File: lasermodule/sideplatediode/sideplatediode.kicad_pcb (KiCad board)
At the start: 2 copper layers, 117 x 33.2 mm, 8 parts, among them J1 Conn_01x02, J2 Conn_01x01, J3 Conn_01x01, J4 Conn_01x01, J5 Conn_01x01

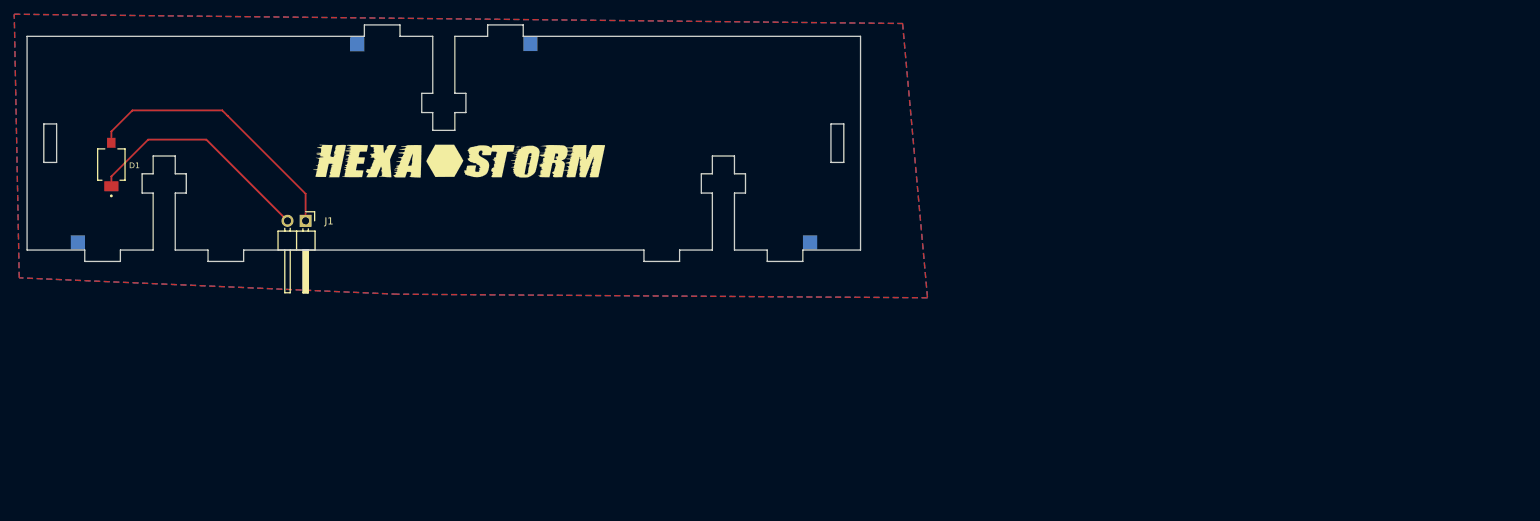
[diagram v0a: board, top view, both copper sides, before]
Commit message: board almost fully synced close for release
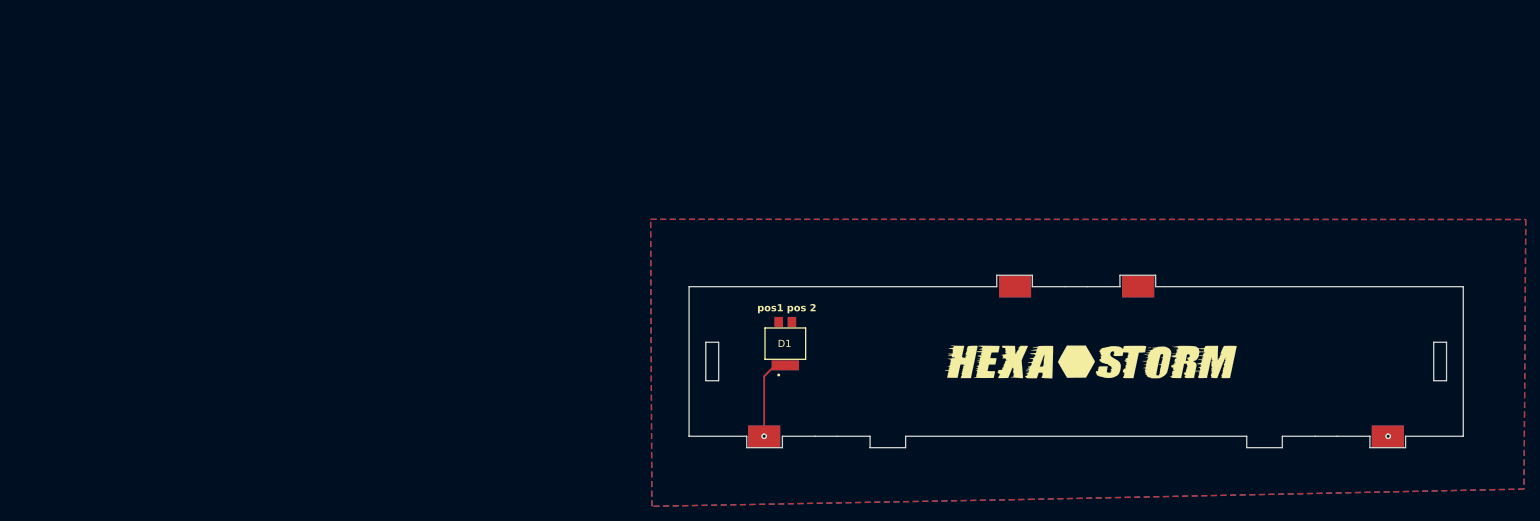
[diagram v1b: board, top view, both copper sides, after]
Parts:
- removed J1: Conn_01x02, Connector_PinHeader_2.54mm:PinHeader_1x02_P2.54mm_Horizontal
- J2, J3, J4, J5, L1: moved to F.Cu
- L2: moved to B.Cu
- moved J5 100.1 mm to (107.2, 111.5), turned to 0 degrees
- moved J2 98.4 mm to (142.4, 90.5), turned to 0 degrees
- moved D1 97.0 mm to (109.2, 98.5)
- moved L1 96.8 mm to (153.0, 101.0), turned to 0 degrees
- moved J3 91.9 mm to (159.7, 90.5), turned to 0 degrees
- moved L2 89.3 mm to (149.1, 101.0), turned to 180 degrees
- moved J4 85.6 mm to (194.8, 111.5), turned to 0 degrees
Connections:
- D1 pad A: Net-(J1-Pin_1) -> GND
- D1 pad C: Net-(J1-Pin_2) -> DiodeK
- J4 pad 1: unconnected-(J4-Pin_1-Pad1) -> GND
- J5 pad 1: unconnected-(J5-Pin_1-Pad1) -> DiodeK
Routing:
- net Net-(J1-Pin_1): track 38.7 -> 0.00 mm
- net Net-(J1-Pin_2): track 33.0 -> 0.00 mm
- net DiodeK: track 0.00 -> 11.7 mm, vias 0 -> 1
- net GND: vias 0 -> 1
- added copper zone on B.Cu, net GND
- added copper zone on F.Cu, net GND
- removed copper zone on B.Cu, net Net-(J1-Pin_1)
- removed copper zone on F.Cu, net Net-(J1-Pin_1)
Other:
- board size 117 x 33.2 mm -> 108.7 x 24.2 mm
- board text added: "pos 2"
- board text added: "pos1"
